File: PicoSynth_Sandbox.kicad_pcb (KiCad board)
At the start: 2 copper layers, 164 x 75 mm, 0 parts

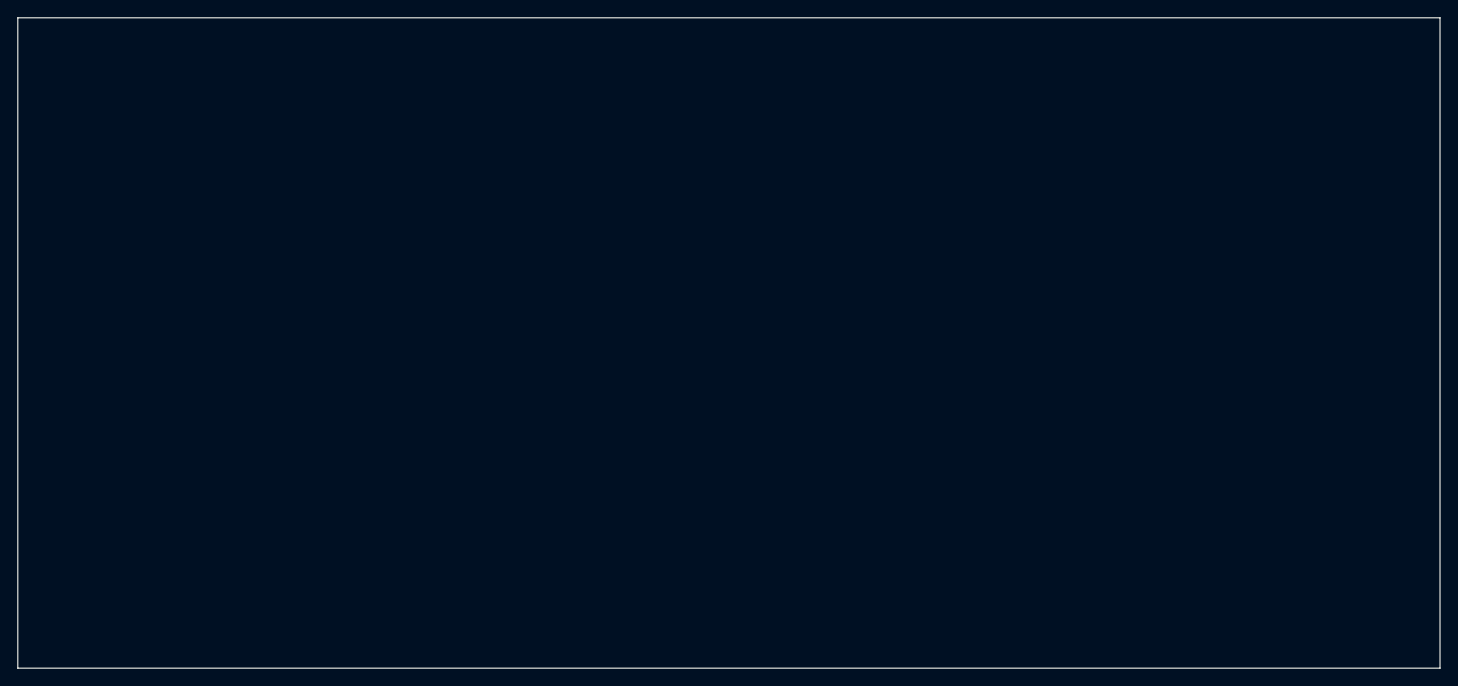
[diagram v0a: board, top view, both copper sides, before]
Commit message: Board outline.
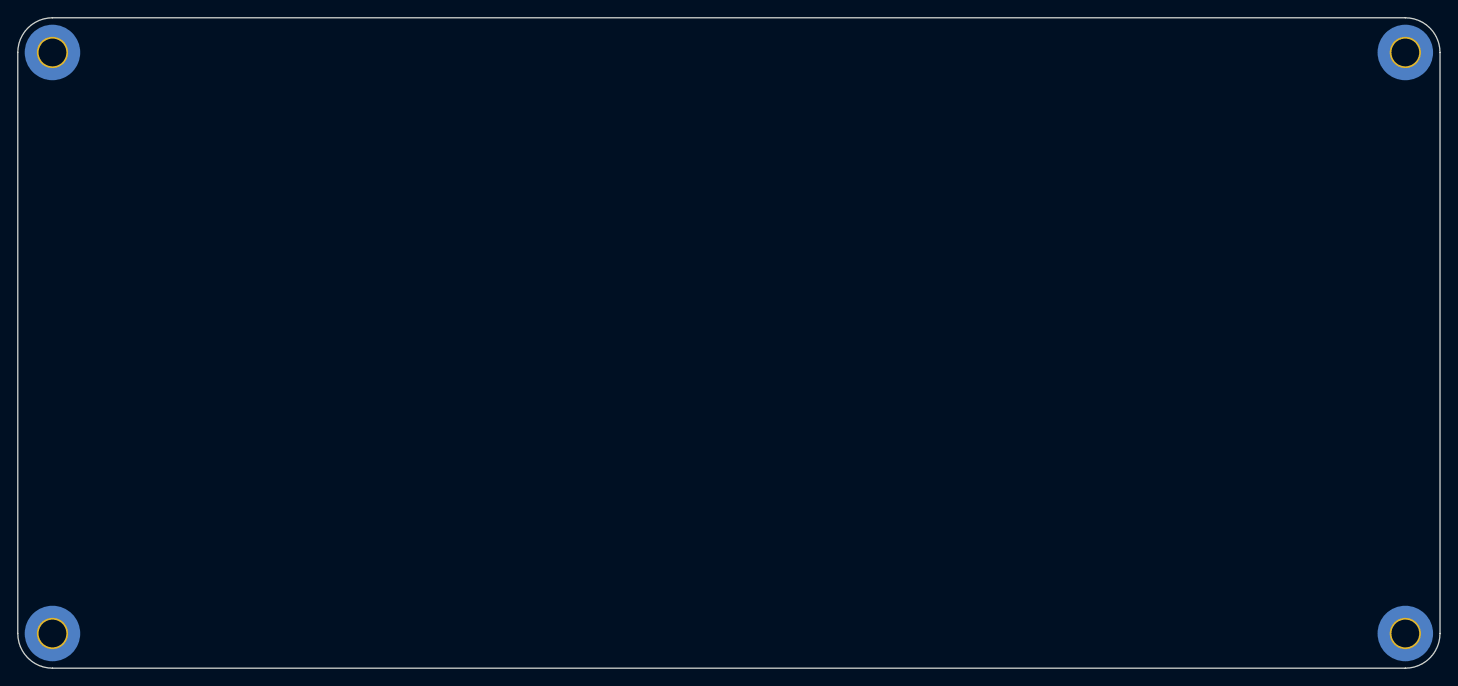
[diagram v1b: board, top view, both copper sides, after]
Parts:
- added H1: MountingHole_Pad, MountingHole:MountingHole_3.2mm_M3_Pad_TopOnly, B.Cu at (70.0, 72.0)
- added H2: MountingHole_Pad, MountingHole:MountingHole_3.2mm_M3_Pad_TopOnly, B.Cu at (226.0, 72.0)
- added H3: MountingHole_Pad, MountingHole:MountingHole_3.2mm_M3_Pad_TopOnly, B.Cu at (226.0, 139.0)
- added H4: MountingHole_Pad, MountingHole:MountingHole_3.2mm_M3_Pad_TopOnly, B.Cu at (70.0, 139.0)
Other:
- outline, holes or cut-outs redrawn
